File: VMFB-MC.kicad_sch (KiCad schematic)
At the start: 44 parts, among them J1 Conn_01x04_Pin, J10 Conn_01x04_Pin, J2 Conn_01x04_Pin, J3 Conn_01x04_Pin, J4 Conn_01x02_Pin, J5 Conn_01x03_Pin, J6 Conn_01x04_Pin, J7 Conn_01x04_Pin, J8 Conn_01x04_Pin, J9 Conn_01x05_Pin, Q1 SFH313FA-2/3, Q2 SFH313FA-2/3, Q3 SFH313FA-2/3, Q4 SFH313FA-2/3, Q5 SFH313FA-2/3, Q6 SFH313FA-2/3, Q7 TIP120, Q8 TIP120, Q9 SFH313FA-2/3, U1 LM393

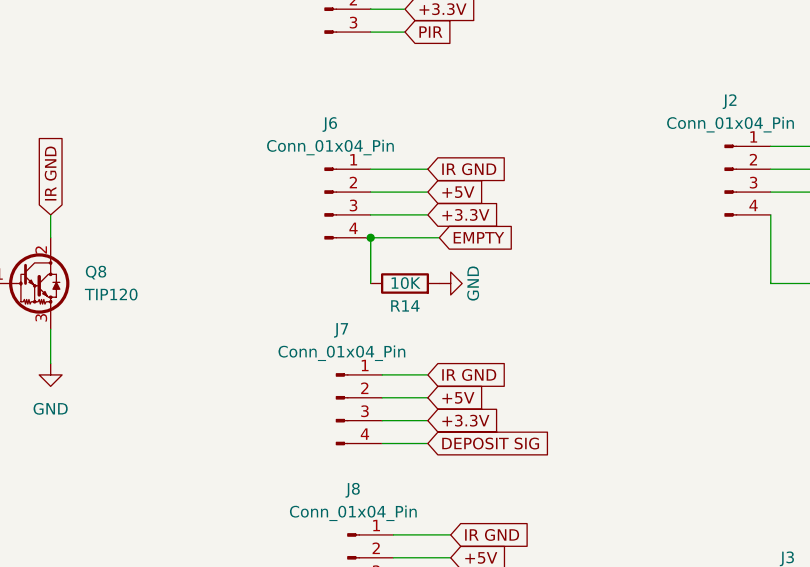
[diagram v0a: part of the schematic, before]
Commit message: more clean up
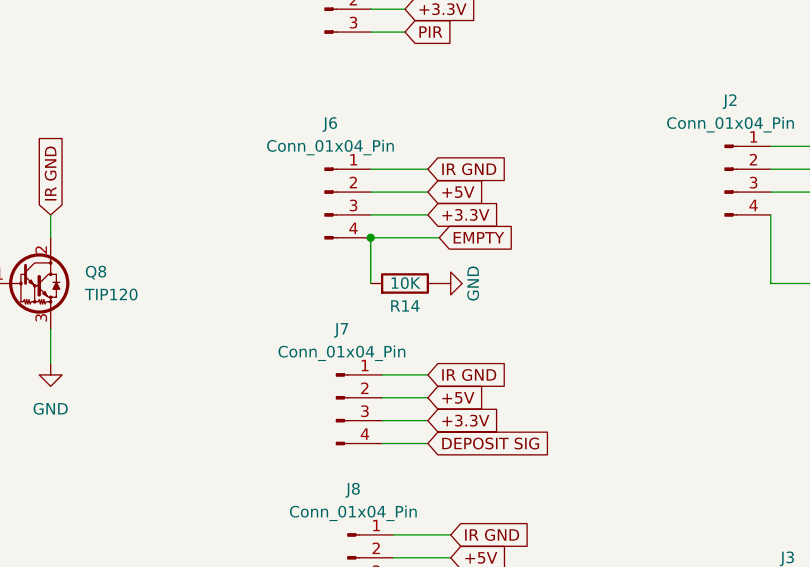
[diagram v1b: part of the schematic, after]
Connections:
- net EMPTY: now also R14.2; no longer R14.1
- net GND: now also R14.1; no longer R14.2
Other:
- moved on the sheet: R14
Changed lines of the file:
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@@
     )
   )
-  (symbol (lib_id "Device:R") (at 139.7 101.6 90) (unit 1)
+  (symbol (lib_id "Device:R") (at 139.7 101.6 270) (mirror x) (unit 1)
     (in_bom yes) (on_board yes) (dnp no)
     (property "Reference" "R14" (at 139.7 104.14 90)
